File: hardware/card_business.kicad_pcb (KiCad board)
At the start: 2 copper layers, 49.9 x 17.3 mm, 12 parts, among them J1 Conn_01x01_Female, J2 USB_A, SW1 Reset, SW2 Boot, U1 CH552G

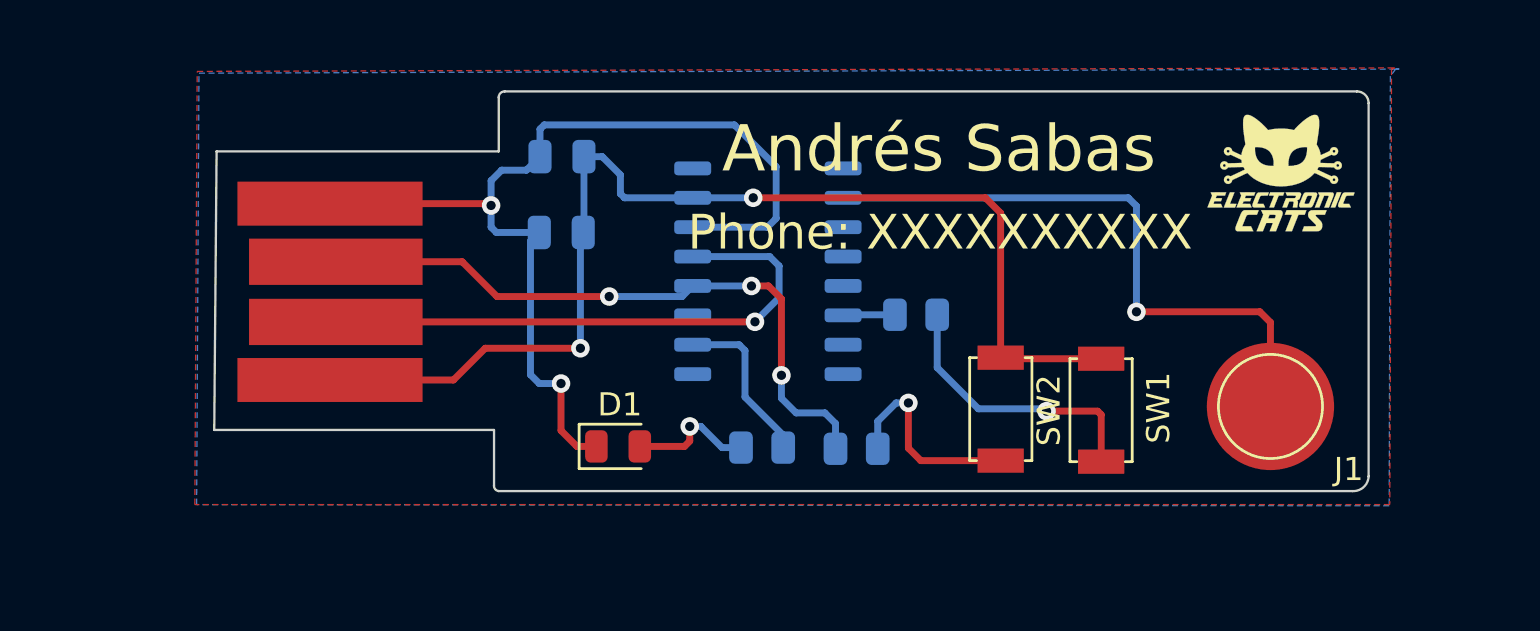
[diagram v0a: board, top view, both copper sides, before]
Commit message: Change pin name and routing update
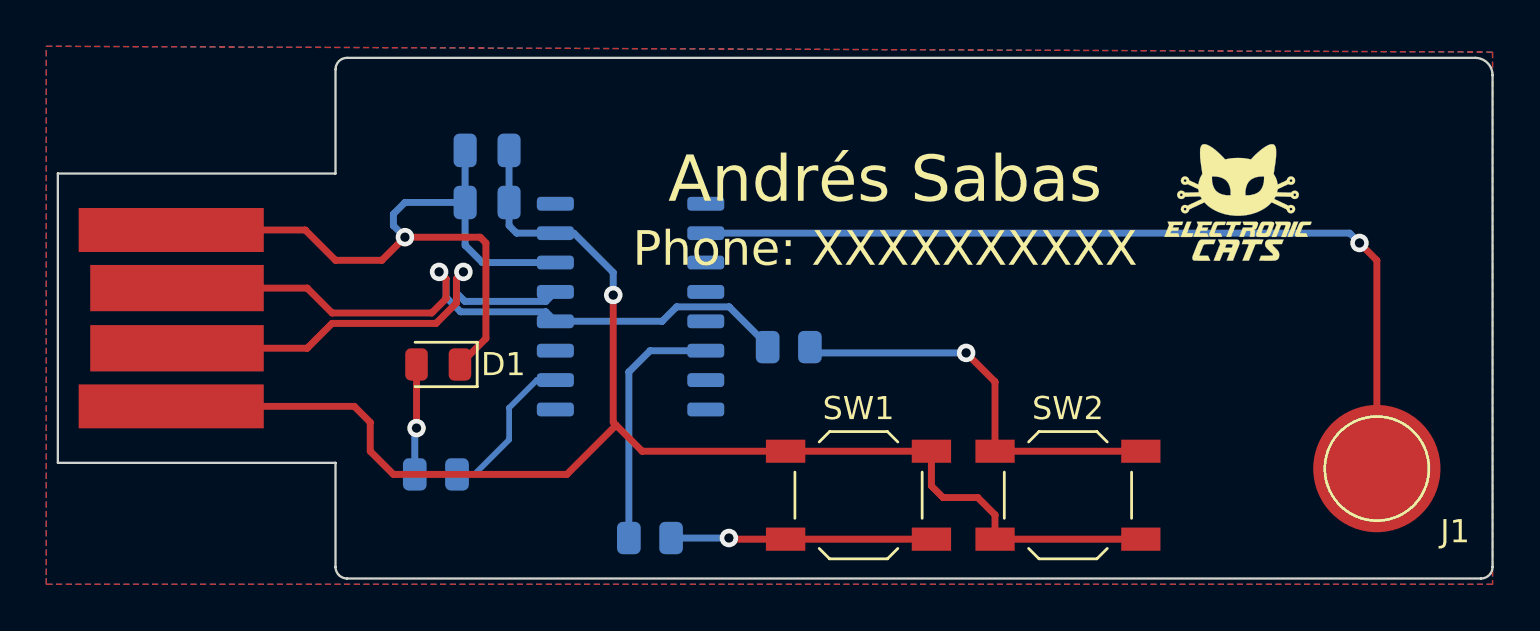
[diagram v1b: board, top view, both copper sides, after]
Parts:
- SW1, SW2: footprint Connectors:C455281 -> Button_Switch_SMD:SW_SPST_TL3342
- moved R1 15.0 mm to (105.1, 95.5)
- moved R3 14.1 mm to (95.8, 92.8)
- moved SW1 13.2 mm to (114.1, 93.7), turned to 0 degrees
- moved D1 8.54 mm to (95.9, 88.0), turned to 180 degrees
- moved J2 6.96 mm to (79.5, 86.0)
- moved U1 6.13 mm to (104.2, 85.5)
- moved J1 5.32 mm to (136.5, 92.5)
- moved R2 5.28 mm to (111.1, 87.2)
- moved SW2 4.50 mm to (123.2, 93.7), turned to 0 degrees
- moved C1 3.46 mm to (98.0, 81.0)
- moved C2 3.25 mm to (98.0, 78.8)
- moved G*** 2.25 mm to (130.5, 81.0)
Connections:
- net /UDM renamed /UD-
- net /UDP renamed /UD+
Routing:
- net +5V: track 49.8 -> 64.0 mm, vias 2 -> 1
- net /PAD: track 27.0 -> 38.5 mm
- net GND: track 43.6 -> 33.2 mm, vias 2 -> 1
- net Net-(R2-Pad1): track 9.01 -> 17.9 mm
- net /RST: track 2.25 -> 10.9 mm
- net /UD-: track 24.9 -> 20.0 mm
- net /UD+: track 28.5 -> 30.2 mm, vias 3 -> 1
- net /P3.3: track 7.80 -> 6.74 mm
- net Net-(R1-Pad2): track 12.2 -> 11.3 mm
- net Net-(D1-Pad2): track 5.48 -> 4.78 mm
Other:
- board size 49.9 x 17.3 mm -> 62 x 22.5 mm
